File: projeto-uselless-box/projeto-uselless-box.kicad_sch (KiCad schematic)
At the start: 11 parts, among them M1 Motor_Servo, M2 Motor_Servo, M3 Motor_Servo, M4 Fita de Led, Q1 BC337, SW1 SW_DPST_x2, U3 L7812

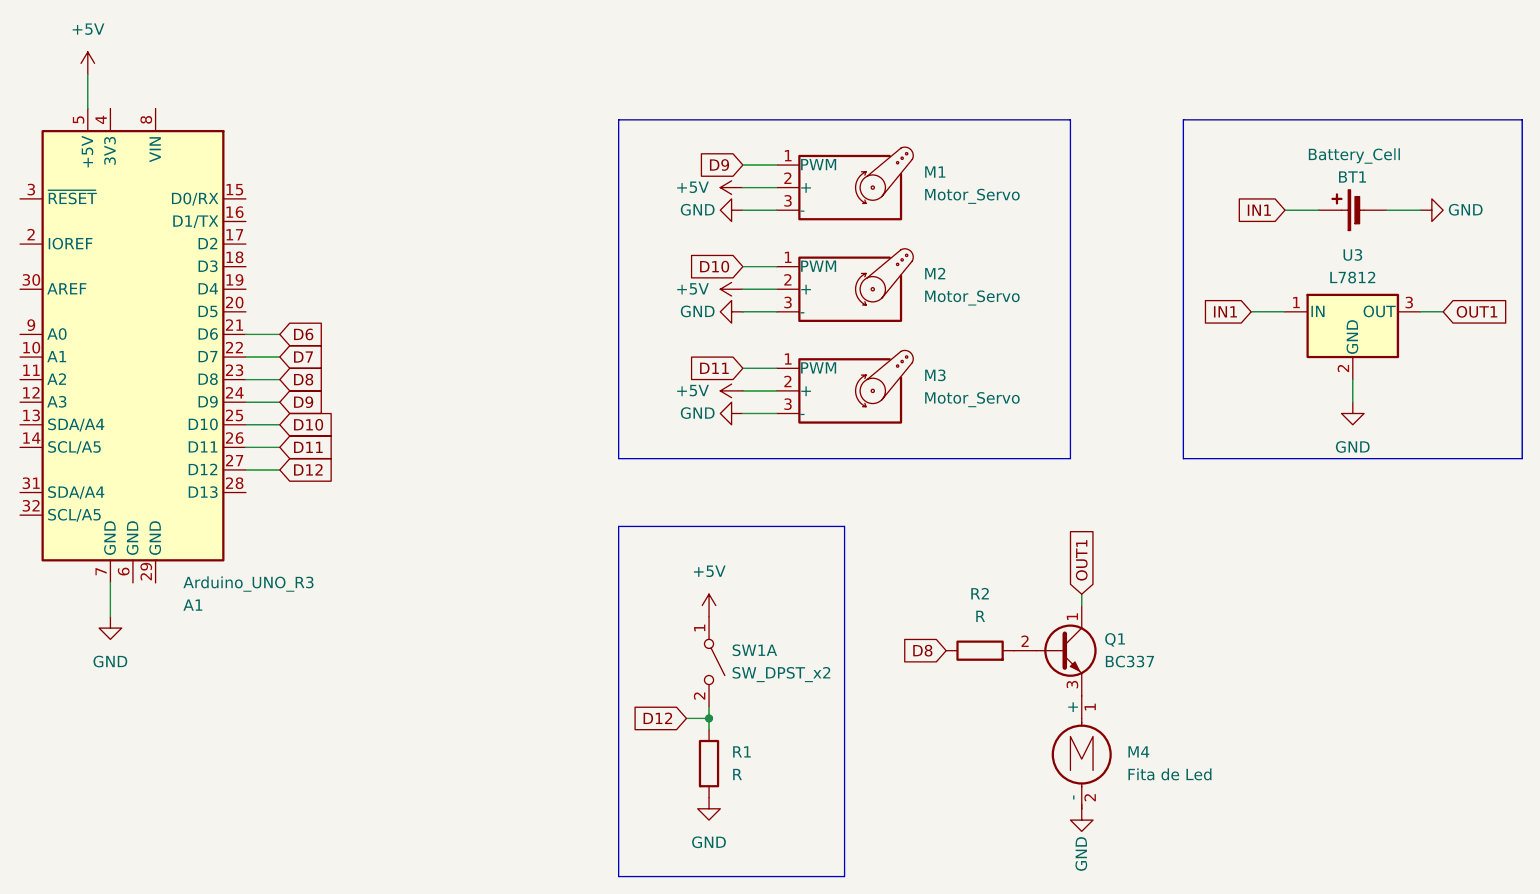
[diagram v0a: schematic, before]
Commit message: Fixing some things
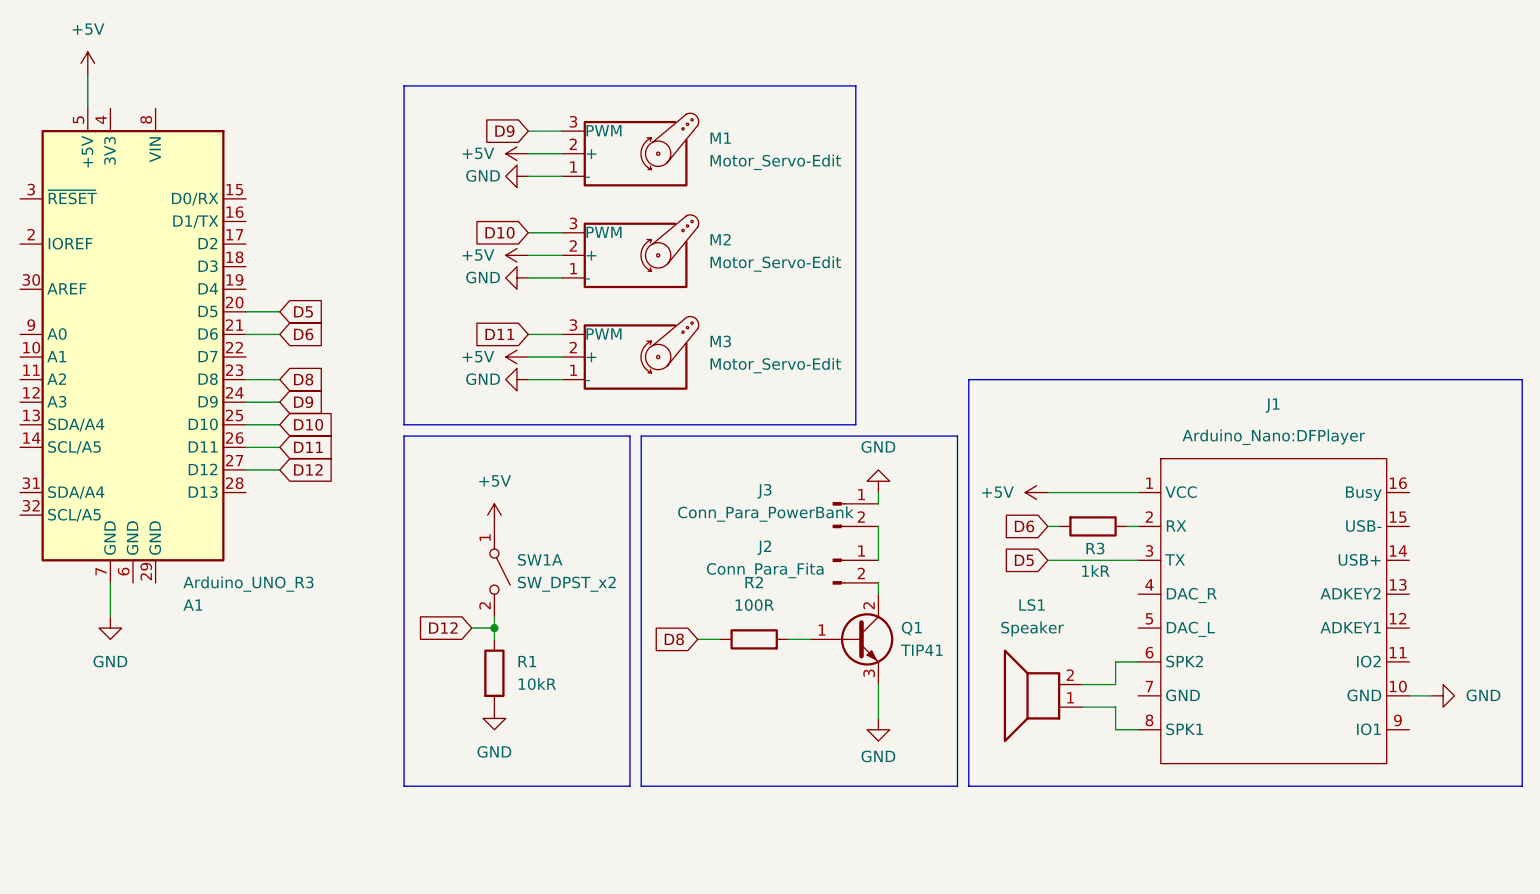
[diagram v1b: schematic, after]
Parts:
- removed BT1: Battery_Cell, symbol Device:Battery_Cell
- removed M1, M2, M3: Motor_Servo, symbol Motor:Motor_Servo
- removed M4: Fita de Led, symbol Motor:Motor_DC
- removed Q1: BC337, Package_TO_SOT_THT:TO-92_Inline, symbol Transistor_BJT:BC337
- removed U3: L7812, symbol Regulator_Linear:L7812
- added J1: ~, Arduino_Nano:DFPlayer, symbol Arduino_Nano:DFPlayer
- added J2: Conn_Para_Fita, TerminalBlock_Phoenix:TerminalBlock_Phoenix_MKDS-1,5-2-5.08_1x02_P5.08mm_Horizontal, symbol Connector:Conn_01x02_Pin
- added J3: Conn_Para_PowerBank, TerminalBlock_Phoenix:TerminalBlock_Phoenix_MKDS-1,5-2-5.08_1x02_P5.08mm_Horizontal, symbol Connector:Conn_01x02_Pin
- added LS1: Speaker, TerminalBlock_Phoenix:TerminalBlock_Phoenix_MKDS-1,5-2-5.08_1x02_P5.08mm_Horizontal, symbol Device:Speaker
- added M1, M2, M3: Motor_Servo-Edit, Connector_PinSocket_2.54mm:PinSocket_1x02_P2.54mm_Vertical, symbol New_Library:Motor_Servo-Edit
- added Q1: TIP41, Package_TO_SOT_THT:TO-220-3_Vertical, symbol Transistor_BJT:TIP41
- added R3: 1kR, Resistor_THT:R_Axial_DIN0207_L6.3mm_D2.5mm_P10.16mm_Horizontal, symbol Device:R
- R1: value R -> 10kR; footprint (none) -> Resistor_THT:R_Axial_DIN0207_L6.3mm_D2.5mm_P10.16mm_Horizontal
- R2: value R -> 100R; footprint (none) -> Resistor_THT:R_Axial_DIN0207_L6.3mm_D2.5mm_P10.16mm_Horizontal
- SW1: footprint (none) -> TerminalBlock_Phoenix:TerminalBlock_Phoenix_MKDS-1,5-2-5.08_1x02_P5.08mm_Horizontal
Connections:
- net +5V: now also J1.1 (VCC), M1.2 (+), M2.2 (+), M3.2 (+)
- net D10: now also M2.3 (PWM)
- net D11: now also M3.3 (PWM)
- net D6: now also R3.2
- net D9: now also M1.3 (PWM)
- net GND: now also J1.10 (GND), J3.1 (Pin_1), M1.1 (-), M2.1 (-), M3.1 (-), Q1.3 (E)
- net at R2.2: now also Q1.1 (B)
- net D5: now reaches A1.20 (D5)
- net D5: now also J1.3 (TX)
- net D7: no longer names the net of A1.22 (D7)
- new net: J1.2 (RX), R3.1
- new net: J1.8 (SPK1), LS1.1
- new net: J1.6 (SPK2), LS1.2
- new net: J2.2 (Pin_2), Q1.2 (C)
- new net: J2.1 (Pin_1), J3.2 (Pin_2)
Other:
- moved on the sheet: R1, SW1A
